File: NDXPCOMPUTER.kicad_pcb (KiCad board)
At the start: 2 copper layers, 5 parts, among them U1 STM32H723VGTx, U2 BMI088, U3 LSM6DSM, U4 BMP280, U5 NEO-M9N

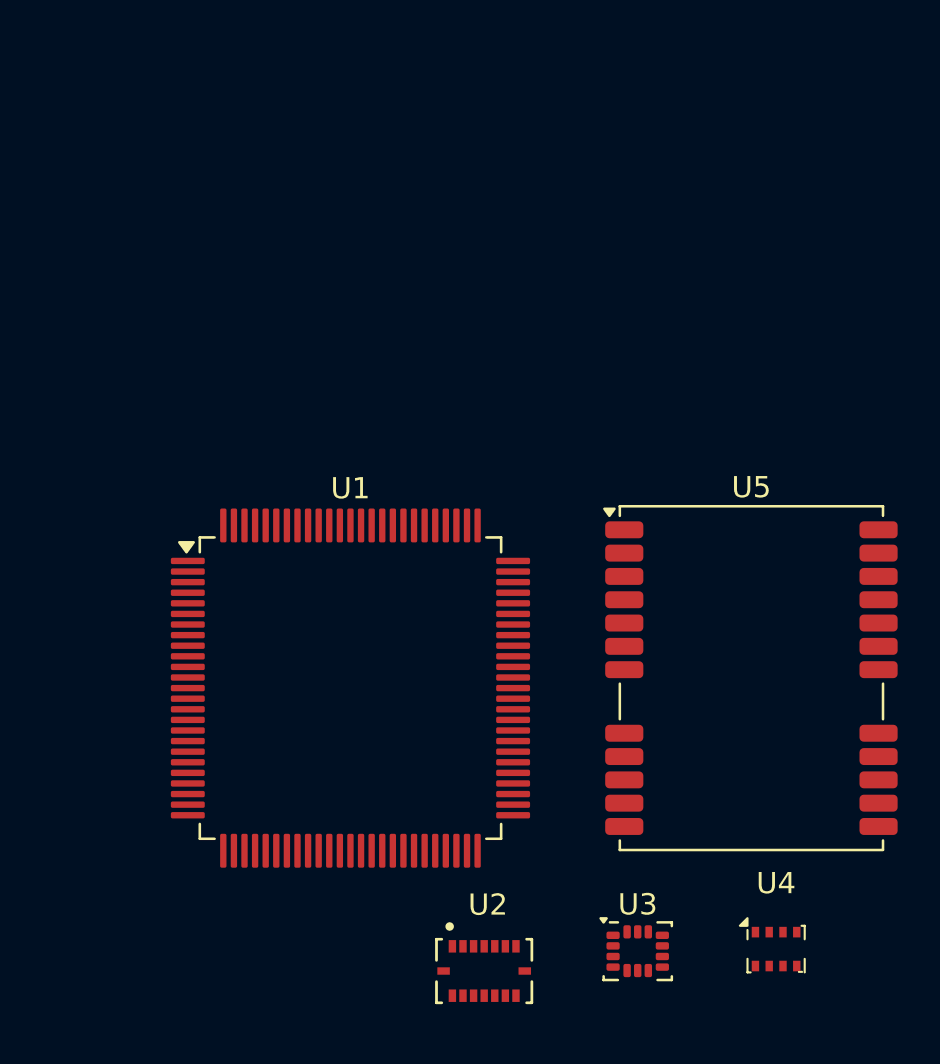
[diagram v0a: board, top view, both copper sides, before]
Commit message: board🏄‍♂️
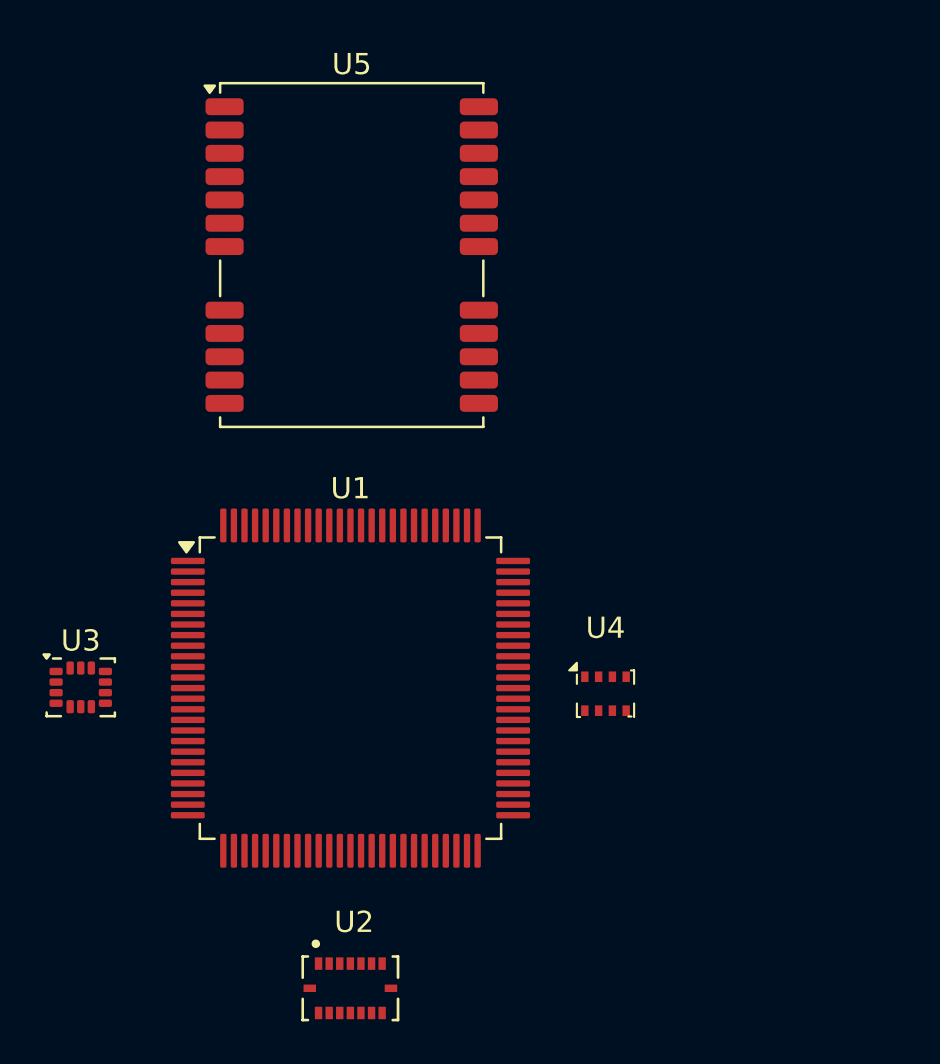
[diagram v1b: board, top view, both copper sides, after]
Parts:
- moved U3 29.1 mm to (127.4, 97.8)
- moved U5 27.5 mm to (140.2, 77.3)
- moved U4 14.5 mm to (152.1, 98.0)
- moved U2 6.37 mm to (140.1, 112.0)
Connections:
- U1 pad 28: unconnected-(U1-PA4-Pad28) -> /BMI088/CS_GYRO
- U1 pad 29: unconnected-(U1-PA5-Pad29) -> /BMI088/SCK
- U1 pad 30: unconnected-(U1-PA6-Pad30) -> /BMI088/SDO_GYRO
- U1 pad 31: unconnected-(U1-PA7-Pad31) -> /BMI088/SDI
- U2 pad 10: unconnected-(U2-SDO2-Pad10) -> /BMI088/SDO_GYRO
- U2 pad 11: unconnected-(U2-VDDIO-Pad11) -> +3.3V
- U2 pad 12: unconnected-(U2-INT3-Pad12) -> /BMI088/GYRO_INT
- U2 pad 14: unconnected-(U2-CSB1-Pad14) -> /BMI088/CS_ACCEL
- U2 pad 15: unconnected-(U2-SDO1-Pad15) -> /BMI088/SDO_ACCEL
- U2 pad 16: unconnected-(U2-INT1-Pad16) -> /BMI088/ACCEL_INT
- U2 pad 2: unconnected-(U2-NC-Pad2) -> GND
- U2 pad 3: unconnected-(U2-VDD-Pad3) -> +3.3V
- U2 pad 4: unconnected-(U2-GNDA-Pad4) -> GND
- U2 pad 5: unconnected-(U2-CSB2-Pad5) -> /BMI088/CS_GYRO
- U2 pad 6: unconnected-(U2-GNDIO-Pad6) -> GND
- U2 pad 7: unconnected-(U2-PS-Pad7) -> GND
- U2 pad 8: unconnected-(U2-SCL/SCK-Pad8) -> /BMI088/SCK
- U2 pad 9: unconnected-(U2-SDA/SDI-Pad9) -> /BMI088/SDI
